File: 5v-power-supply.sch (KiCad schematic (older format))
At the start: 29 parts

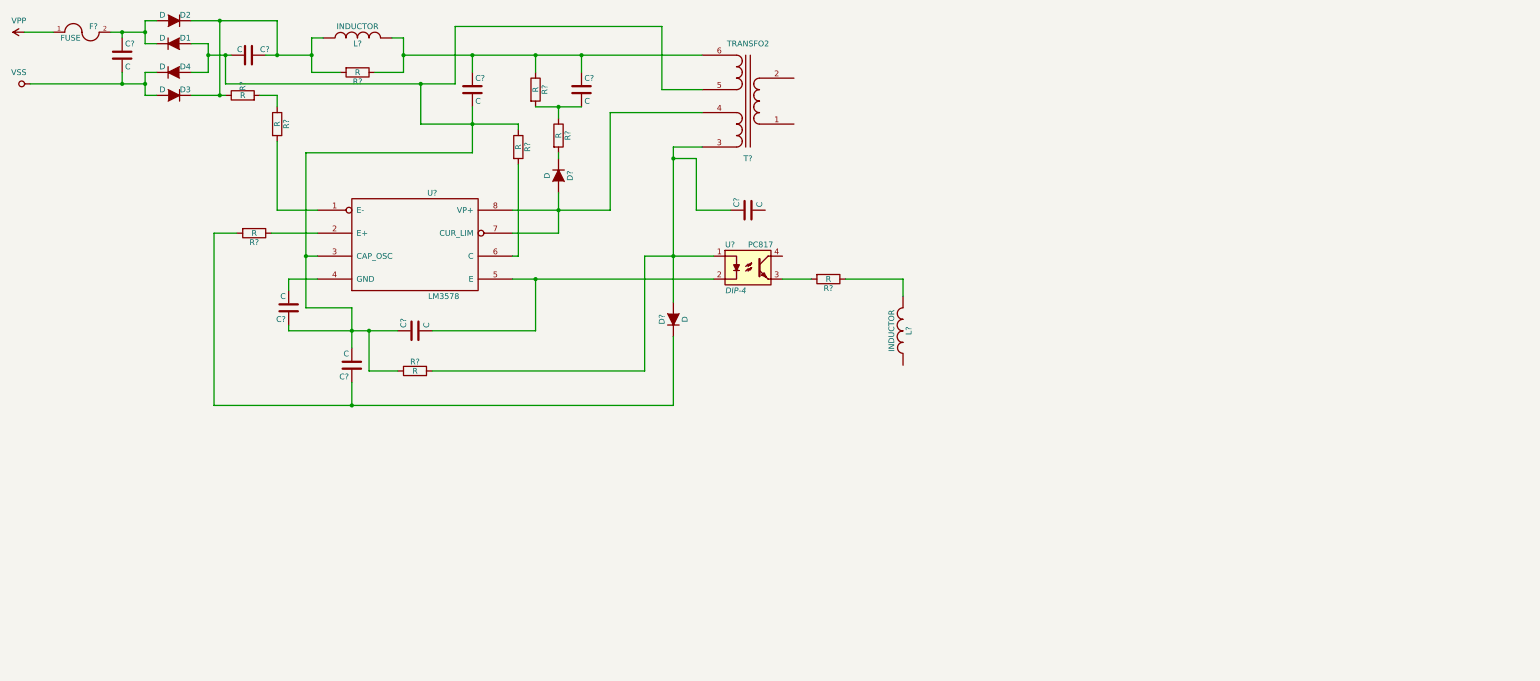
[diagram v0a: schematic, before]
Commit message: the
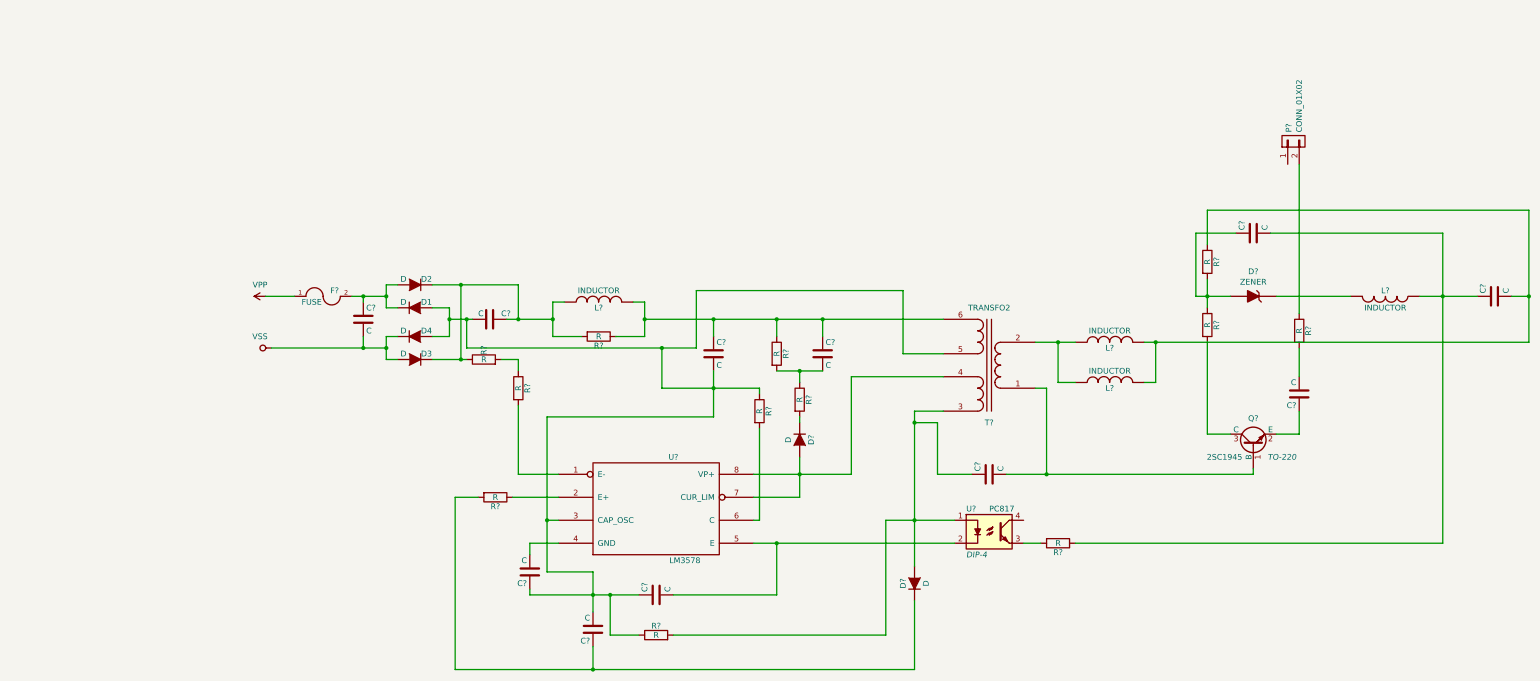
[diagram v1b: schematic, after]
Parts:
- added C? (x3): C, symbol C
- added D?: ZENER, symbol ZENER
- added L? (x2): INDUCTOR, symbol INDUCTOR
- added P?: CONN_01X02, symbol CONN_01X02
- added Q?: 2SC1945, TO-220, symbol 2SC1945
- added R? (x3): R, symbol R
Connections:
- net at T?.1 (AA): now also C?.2, Q?.1 (B)
- net at T?.2 (AB): now also L?.1, L?.1
- net at R?.1: now also C?.1, C?.2, L?.1; no longer L?.2
- new net: C?.2, L?.2, L?.2, R?.1
- new net: C?.1, Q?.2 (E)
- new net: Q?.3 (C), R?.2
- new net: C?.1, D?.2 (A), R?.1, R?.2
- new net: C?.2, R?.2
- new net: P?.2 (P2), R?.1
- new net: D?.1 (K), L?.2
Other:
- moved on the sheet: C?, D1, D2, D3, D4, D?, F?, L?, R?, T?, U?
